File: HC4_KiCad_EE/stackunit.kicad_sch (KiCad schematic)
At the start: 12 parts, among them IC8 74HC377

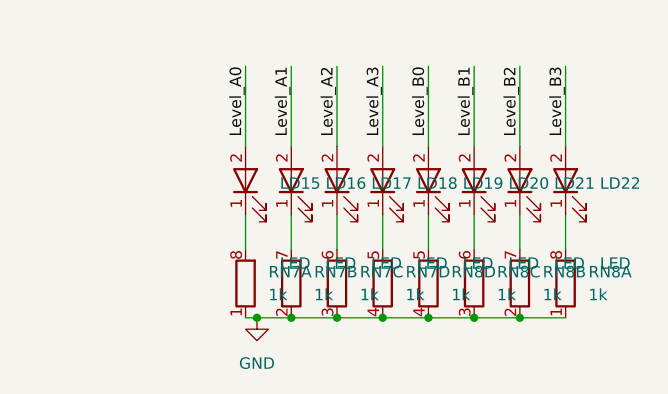
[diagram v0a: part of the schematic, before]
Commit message: 自動配線前最終チェック
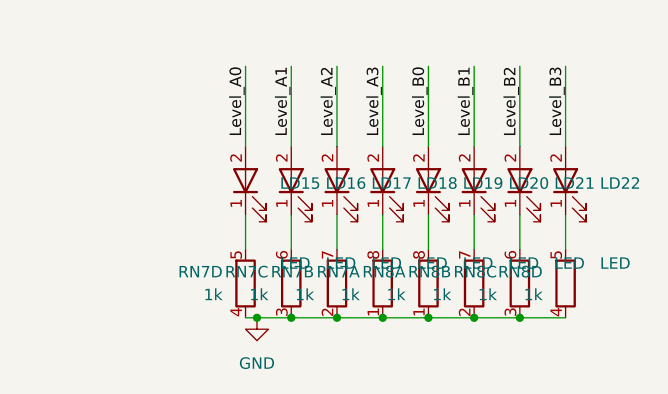
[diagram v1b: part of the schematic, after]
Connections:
- net at RN8.5 (R4.2): now also LD22.1 (K); no longer LD19.1 (K)
- net at LD20.1 (K): now also RN8.7 (R2.2); no longer RN8.6 (R3.2)
- net at RN8.8 (R1.2): now also LD19.1 (K); no longer LD22.1 (K)
- net at RN7.5 (R4.2): now also LD15.1 (K); no longer LD18.1 (K)
- net at LD21.1 (K): now also RN8.6 (R3.2); no longer RN8.7 (R2.2)
- net at RN7.7 (R2.2): now also LD17.1 (K); no longer LD16.1 (K)
- net at RN7.6 (R3.2): now also LD16.1 (K); no longer LD17.1 (K)
- net at RN7.8 (R1.2): now also LD18.1 (K); no longer LD15.1 (K)
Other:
- moved on the sheet: RN7A, RN7B, RN7C, RN7D, RN8A, RN8B, RN8C, RN8D
